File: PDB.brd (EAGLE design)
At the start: 160 x 100 mm, 31 parts, among them J1_CONNECTOR_INPUT 5566-4, U1 MICROCHIP_MIC29300-3_3WUMICRO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, U2 MIC29300-5.0WU-TR

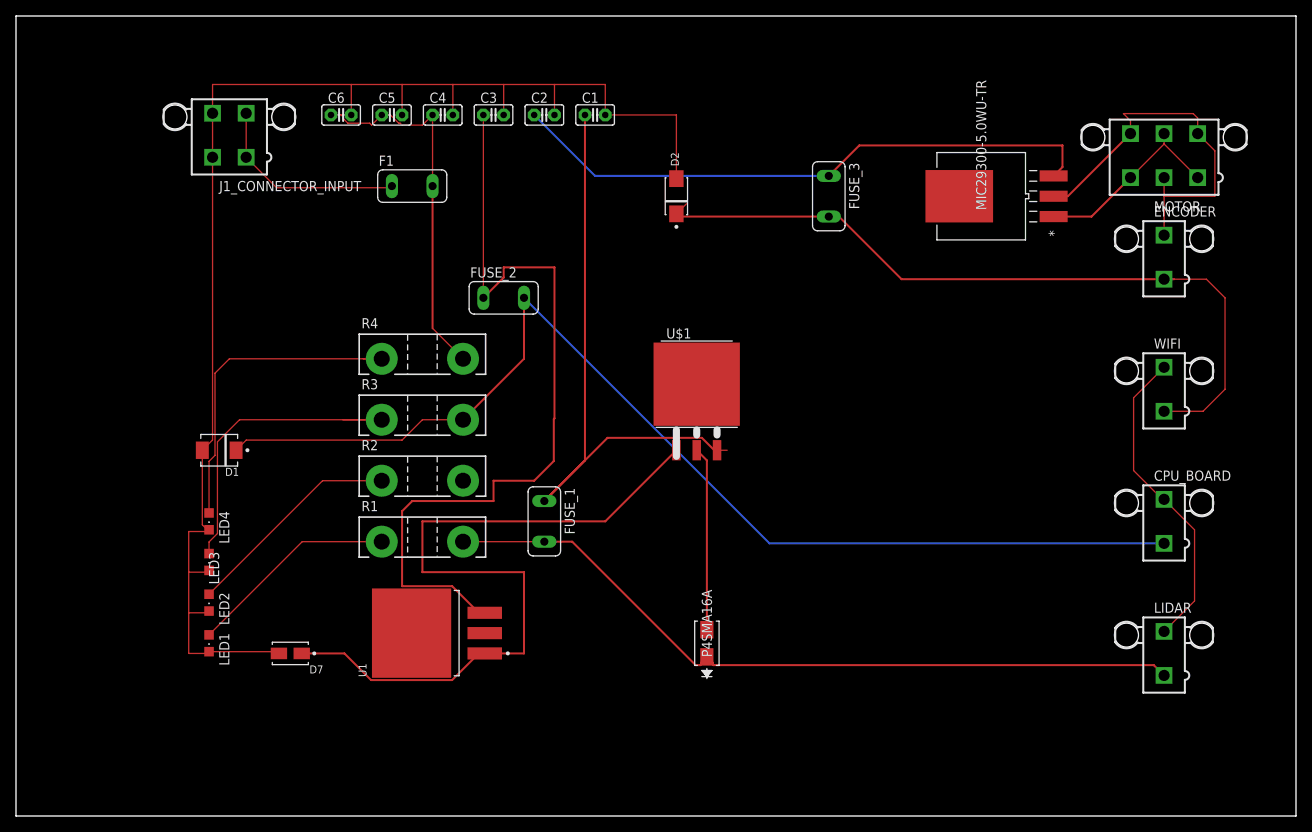
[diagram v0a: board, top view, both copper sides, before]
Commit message: wiring complete
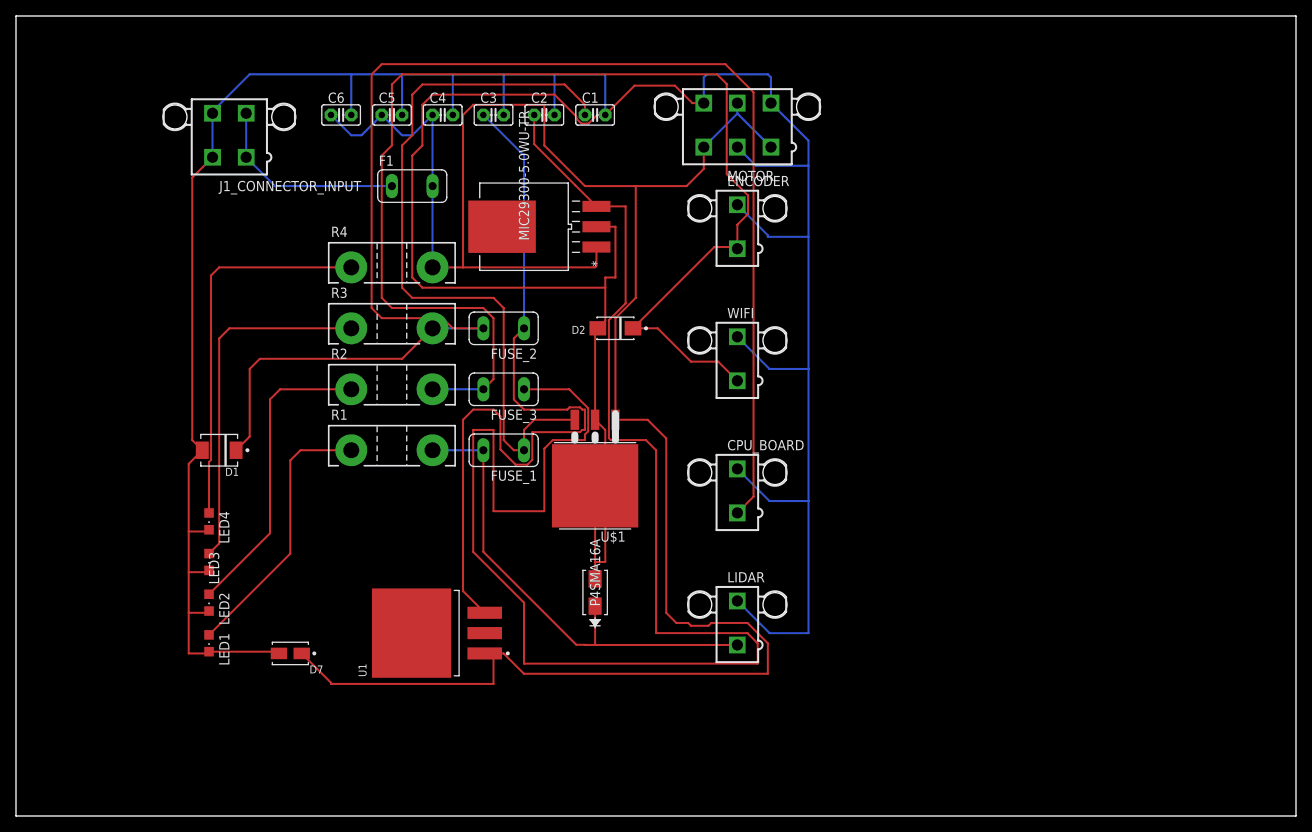
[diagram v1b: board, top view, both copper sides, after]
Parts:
- moved U2 57.3 mm to (63.5, 73.7)
- moved CPU_BOARD 53.5 mm to (90.2, 40.6)
- moved ENCODER 53.5 mm to (90.2, 73.7)
- moved LIDAR 53.5 mm to (90.2, 24.1)
- moved MOTOR 53.5 mm to (90.2, 86.4)
- moved WIFI 53.5 mm to (90.2, 57.1)
- moved FUSE_3 47.3 mm to (61.0, 53.3), turned to 180 degrees
- moved D2 18.2 mm to (74.9, 61.0), turned to 180 degrees
- moved CR1 15.3 mm to (72.4, 27.9)
- moved U$1 13.3 mm to (72.4, 49.5), turned to 180 degrees
- moved R2 12.0 mm to (47.0, 53.3)
- moved R1 12.0 mm to (47.0, 45.7)
- moved R3 12.0 mm to (47.0, 61.0)
- moved R4 12.0 mm to (47.0, 68.6)
- moved FUSE_1 10.2 mm to (61.0, 45.7), turned to 180 degrees
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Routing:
- net GND: track 292.1 -> 452.9 mm
- net N$3: track 75.0 -> 199.9 mm
- net 24V_RAIL: track 167.4 -> 276.2 mm
- net N$6: track 96.2 -> 156.1 mm
- net N$5: track 141.1 -> 189.5 mm
- net N$7: track 95.7 -> 60.5 mm
- net N$1: track 77.1 -> 91.8 mm
- net N$10: track 27.5 -> 38.2 mm
- net N$8: track 26.4 -> 34.2 mm
- net N$2: track 41.7 -> 47.7 mm
- net 2_GND: track 0.00 -> 3.89 mm
- net N$9: track 40.9 -> 44.5 mm
- net N$4: track 102.5 -> 100.5 mm
